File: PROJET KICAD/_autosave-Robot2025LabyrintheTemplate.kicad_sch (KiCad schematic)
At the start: 23 parts, among them J1 HC-SR04 gauche, J10 CAPTEUR TOF _BAS, J11 SERVO MOTEUR 4, J2 +VBatt, J3 SERVO MOTEUR 1, J4 SERVO MOTEUR 2, J5 cap sen0101, J7 SERVO MOTEUR 3, J8 HC-SR04 droite, J9 CAPTEUR TOF_HAUT, U1 module_mpu6050, U3 NRF24L01P-Module-E01ML01DP5_B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

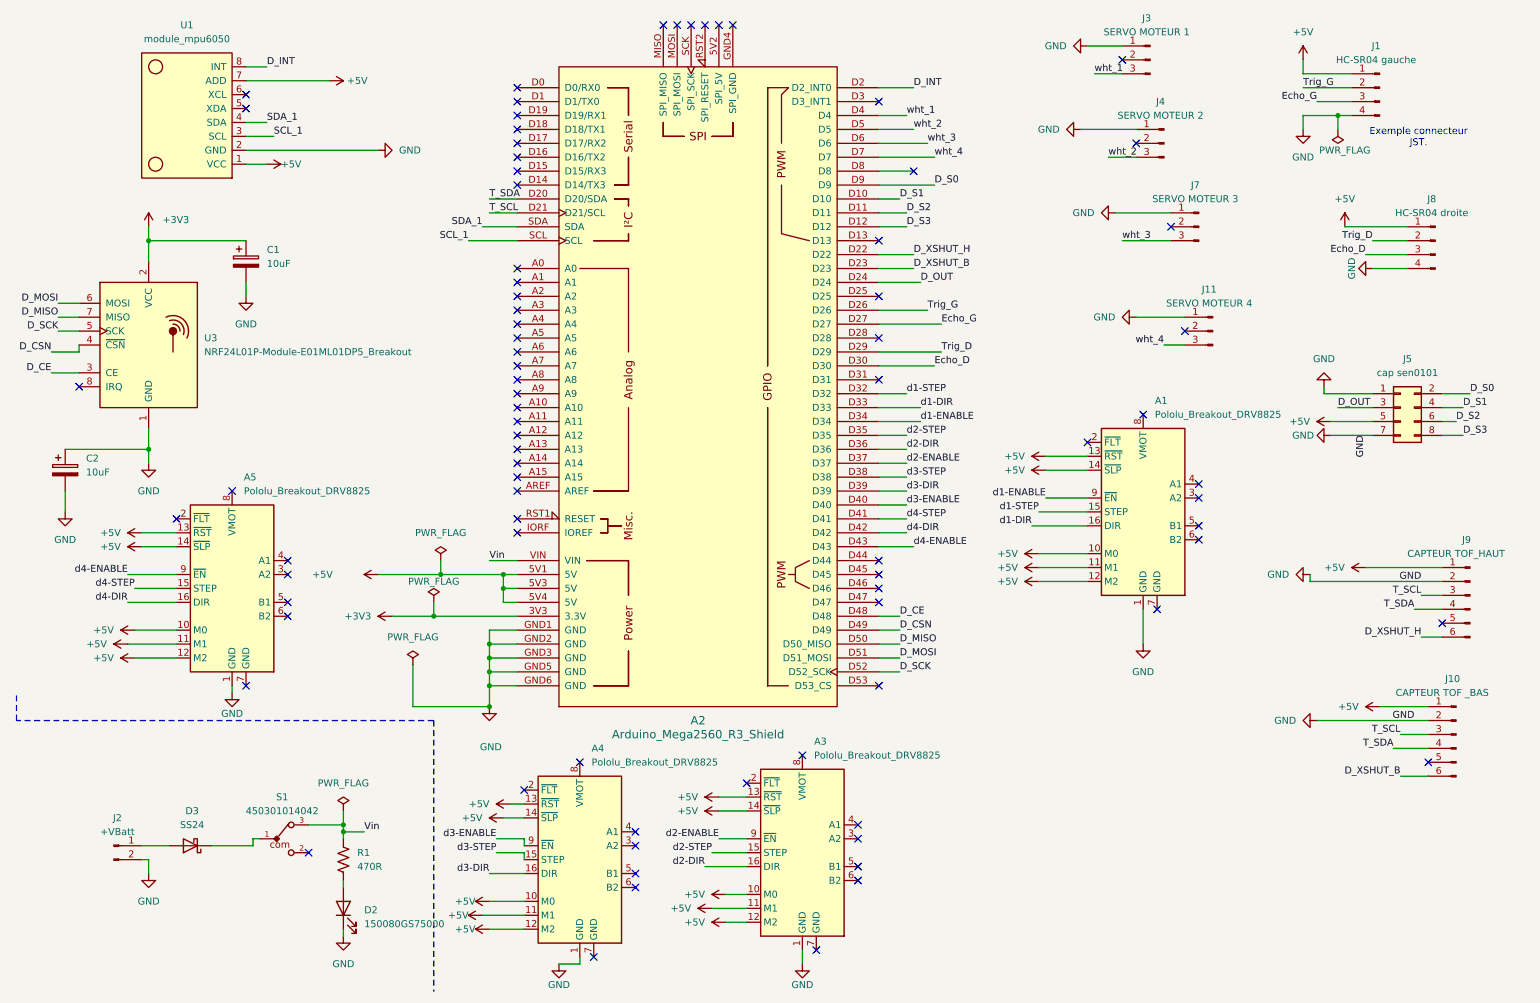
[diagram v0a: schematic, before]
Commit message: revue avec alaime
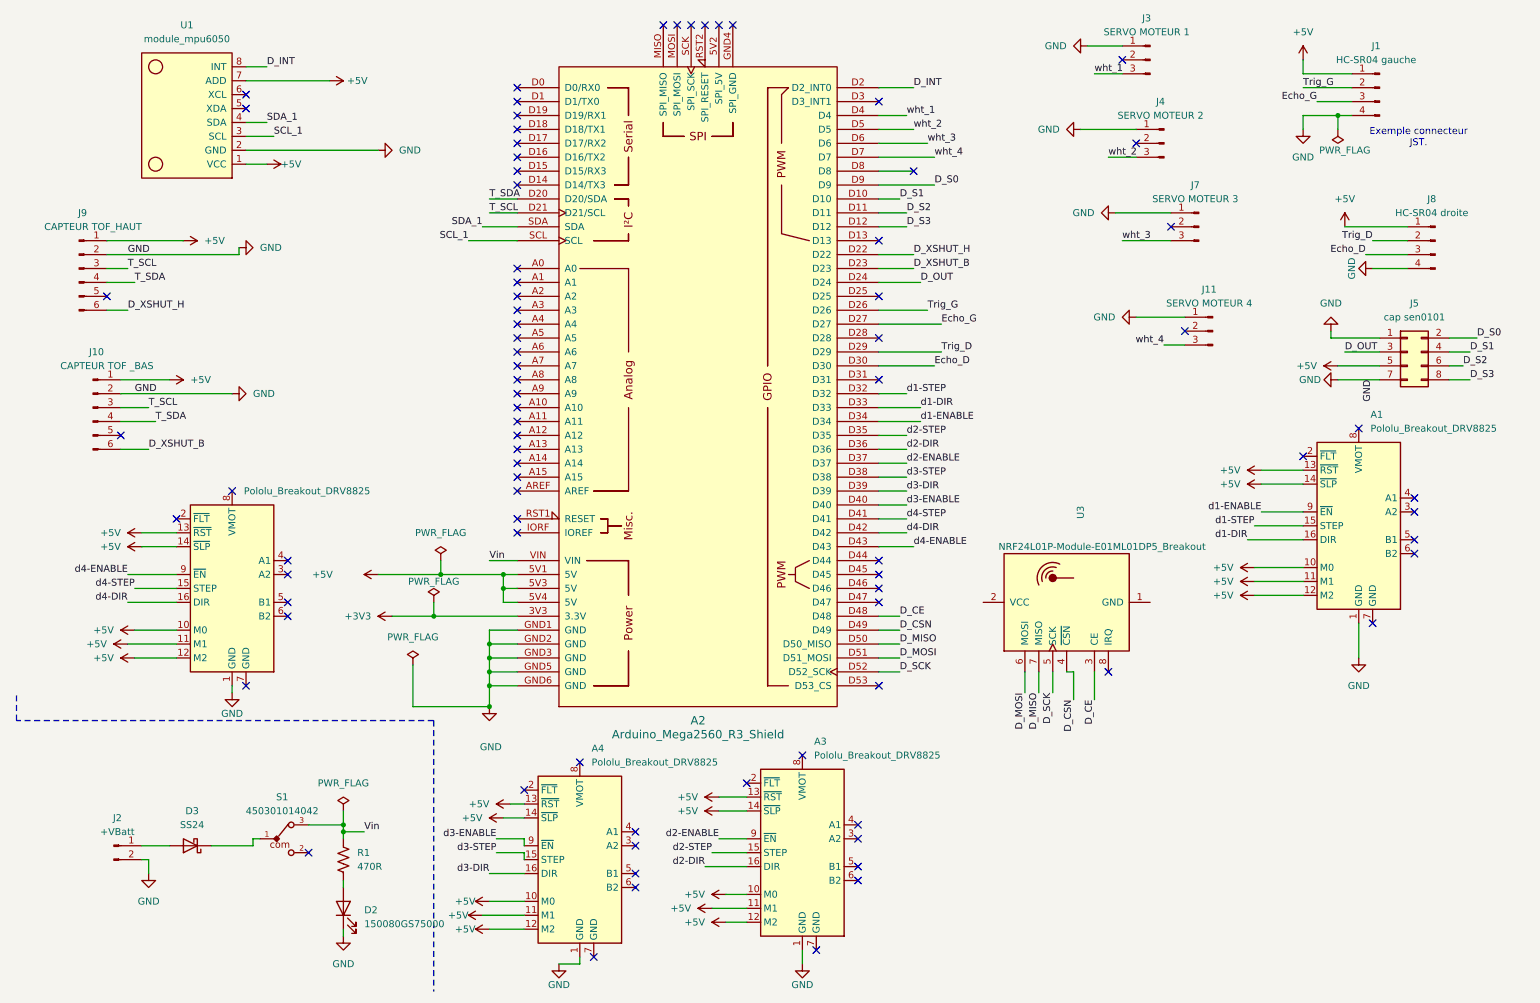
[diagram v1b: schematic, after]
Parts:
- removed C1, C2: 10uF, ISI-Capacitor:WCAP-ATUL_18X35.5_DXL_, symbol ISI-Capacitor:860040781020
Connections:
- net +3V3: no longer U3.2 (VCC)
- net GND: no longer U3.1 (GND)
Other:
- moved on the sheet: A1, J5
